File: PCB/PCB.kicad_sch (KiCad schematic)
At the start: 23 parts, among them J1 Conn_01x06_Pin, U2 A7106, U3 HT7333-3.3V, U4 STM32G031F6Px, Y1 16MHz

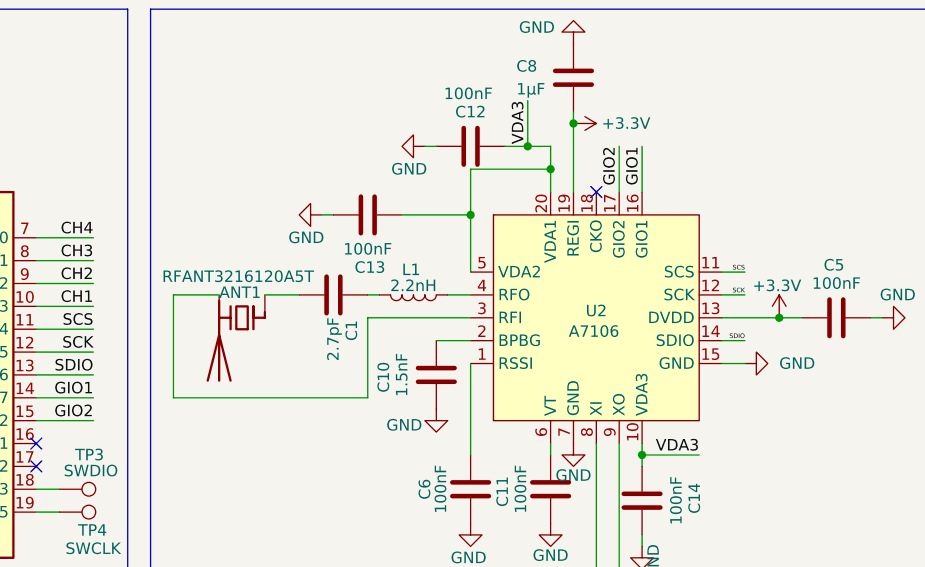
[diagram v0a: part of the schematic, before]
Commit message: Antenna fixes
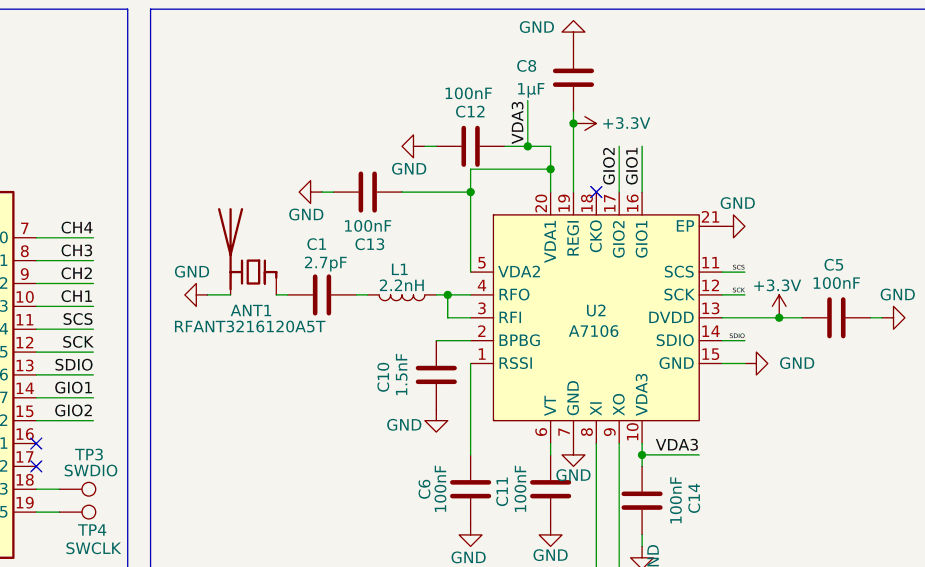
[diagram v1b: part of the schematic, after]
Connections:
- net GND: now also ANT1.2 (PCB_Trace), U2.21 (EP)
- net at U2.3 (RFI): now also L1.1, U2.4 (RFO); no longer ANT1.2 (PCB_Trace)
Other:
- moved on the sheet: ANT1, C1, C13, L1
